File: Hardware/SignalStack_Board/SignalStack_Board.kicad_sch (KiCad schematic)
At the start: 76 parts, among them J2 RJ45_LED_Shielded, J3 Molex_uF_SV_06, Q1 SI4156DY, Q2 SI4156DY, Q3 SI4156DY, Q4 SI4156DY, Q5 SI4156DY, Q6 SI4156DY, Q7 SI4156DY, Q8 SI4156DY, Q9 Q_PMOS_DGS, SW1 SW_Push, SW2 SW_Push, U1 OKI, U10 74LVC2G04, U2 SMAJ12CA, U3 Teensy4.1_DEV-16771, U4 TSR_1-2450, U5 IRS2005S, U6 IRS2005S, U7 74LVC2G04, U8 IRS2005S, U9 IRS2005S

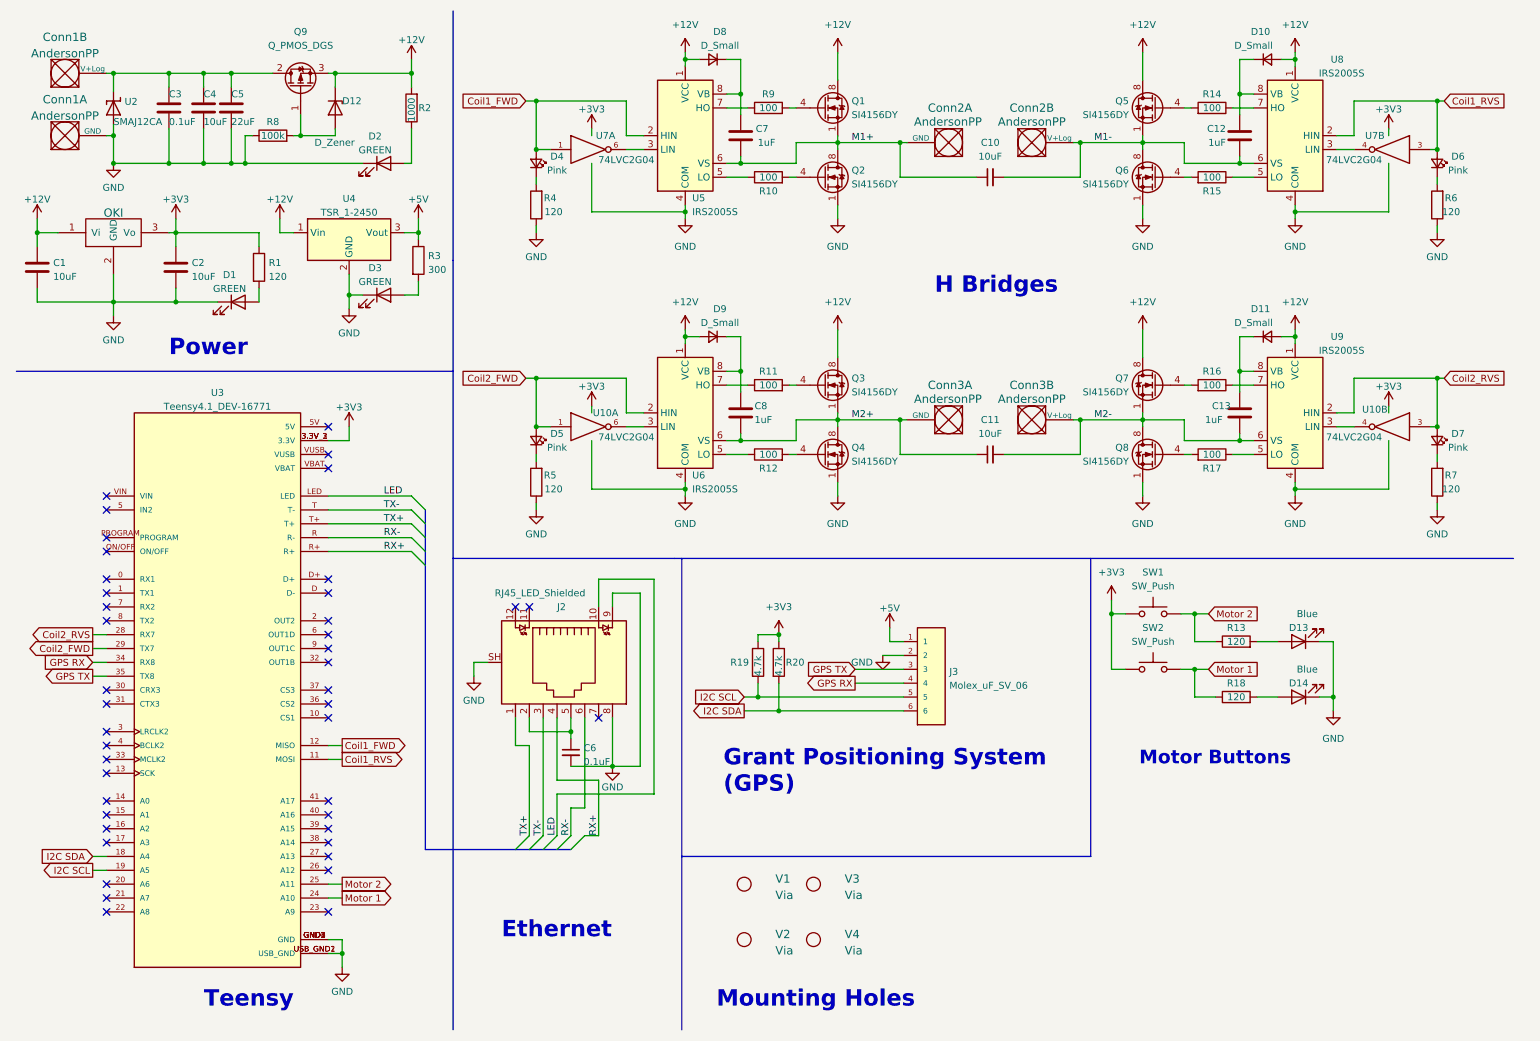
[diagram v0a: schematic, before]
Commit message: Rev3 schematic
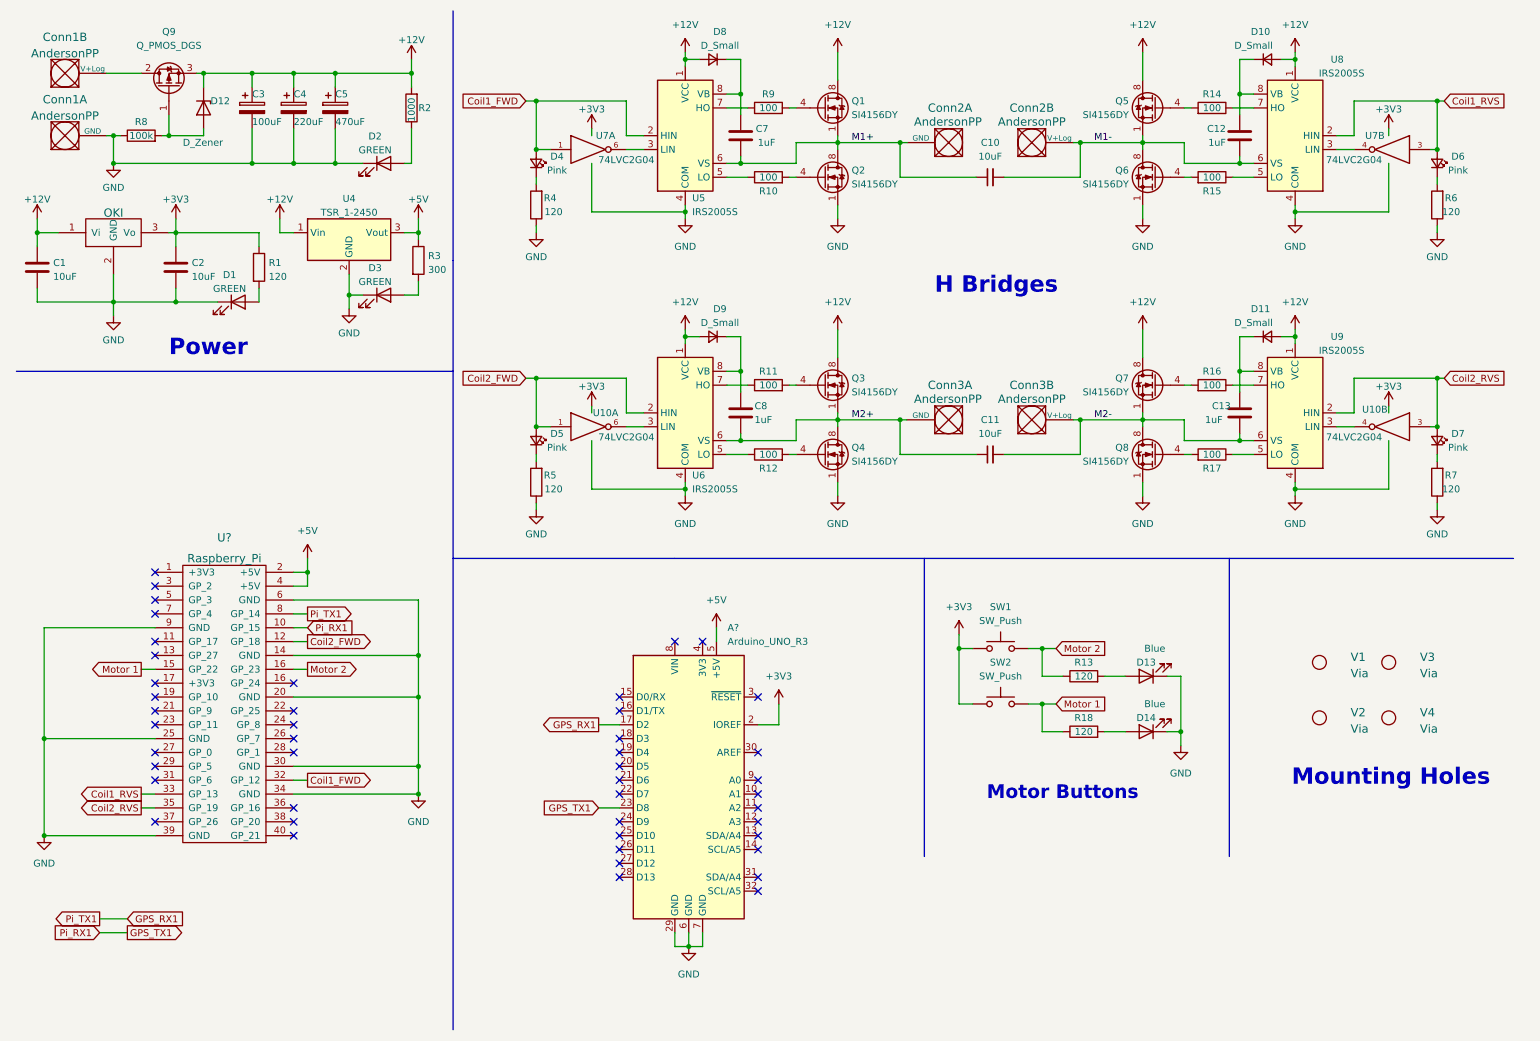
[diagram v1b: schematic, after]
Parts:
- removed C6: 0.1uF, Capacitor_SMD:C_0603_1608Metric_Pad1.08x0.95mm_HandSolder, symbol Device:C_Small
- removed J2: RJ45_LED_Shielded, MRDT_Connectors:RJ45_Teensy, symbol Connector:RJ45_LED_Shielded
- removed J3: Molex_uF_SV_06, Connector_Molex:Molex_SL_171971-0006_1x06_P2.54mm_Vertical, symbol MRDT_Connectors:Molex_uF_SV_06
- removed R19, R20: 4.7k, Resistor_SMD:R_0603_1608Metric_Pad0.98x0.95mm_HandSolder, symbol Device:R
- removed U2: SMAJ12CA, MRDT_Actives:DO-214AC, symbol SMAJ12CA:SMAJ12CA
- removed U3: Teensy4.1_DEV-16771, MRDT_Shields:Teensy_4_1_Ethernet, symbol MRDT_Shields:Teensy4.1_DEV-16771
- added A?: Arduino_UNO_R3, Module:Arduino_UNO_R3, symbol MCU_Module:Arduino_UNO_R3
- added U?: Raspberry_Pi, symbol MRDT_Shields:Raspberry_Pi
- C3: value 0.1uF -> 100uF; symbol Device:C -> Device:C_Polarized
- C4: value 10uF -> 220uF; symbol Device:C -> Device:C_Polarized
- C5: value 22uF -> 470uF; symbol Device:C -> Device:C_Polarized
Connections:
- net +12V: now also C3.1, C4.1, C5.1
- net +3V3: now also A?.2 (IOREF)
- net +5V: now also A?.5 (+5V), U?.2 (+5V), U?.4 (+5V)
- net Coil1_FWD: now also U?.32 (GP_12)
- net Coil1_RVS: now also U?.33 (GP_13)
- net Coil2_FWD: now also U?.12 (GP_18)
- net Coil2_RVS: now also U?.35 (GP_19)
- net GND: now also A?.29 (GND), A?.6 (GND), A?.7 (GND), U?.14 (GND), U?.20 (GND), U?.25 (GND), U?.30 (GND), U?.34 (GND), U?.39 (GND), U?.6 (GND), U?.9 (GND)
- net Motor 1: now also U?.15 (GP_22)
- net Motor 2: now also U?.16 (GP_24)
- new net: Conn1.2 (V+Log), Q9.2 (D)
- new net GPS_RX1: A?.17 (D2), U?.8 (GP_14)
- new net GPS_TX1: A?.23 (D8), U?.10 (GP_15)
- no-connect marks 43 -> 46
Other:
- note removed: "Ethernet"
- note removed: "Grant Positioning System (GPS)"
- note removed: "Teensy"
- moved on the sheet: D12, D13, D14, Q9, R13, R18, R8, SW1, SW2, V1, V2, V3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
